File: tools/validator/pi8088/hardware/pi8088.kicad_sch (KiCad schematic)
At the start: 2 parts

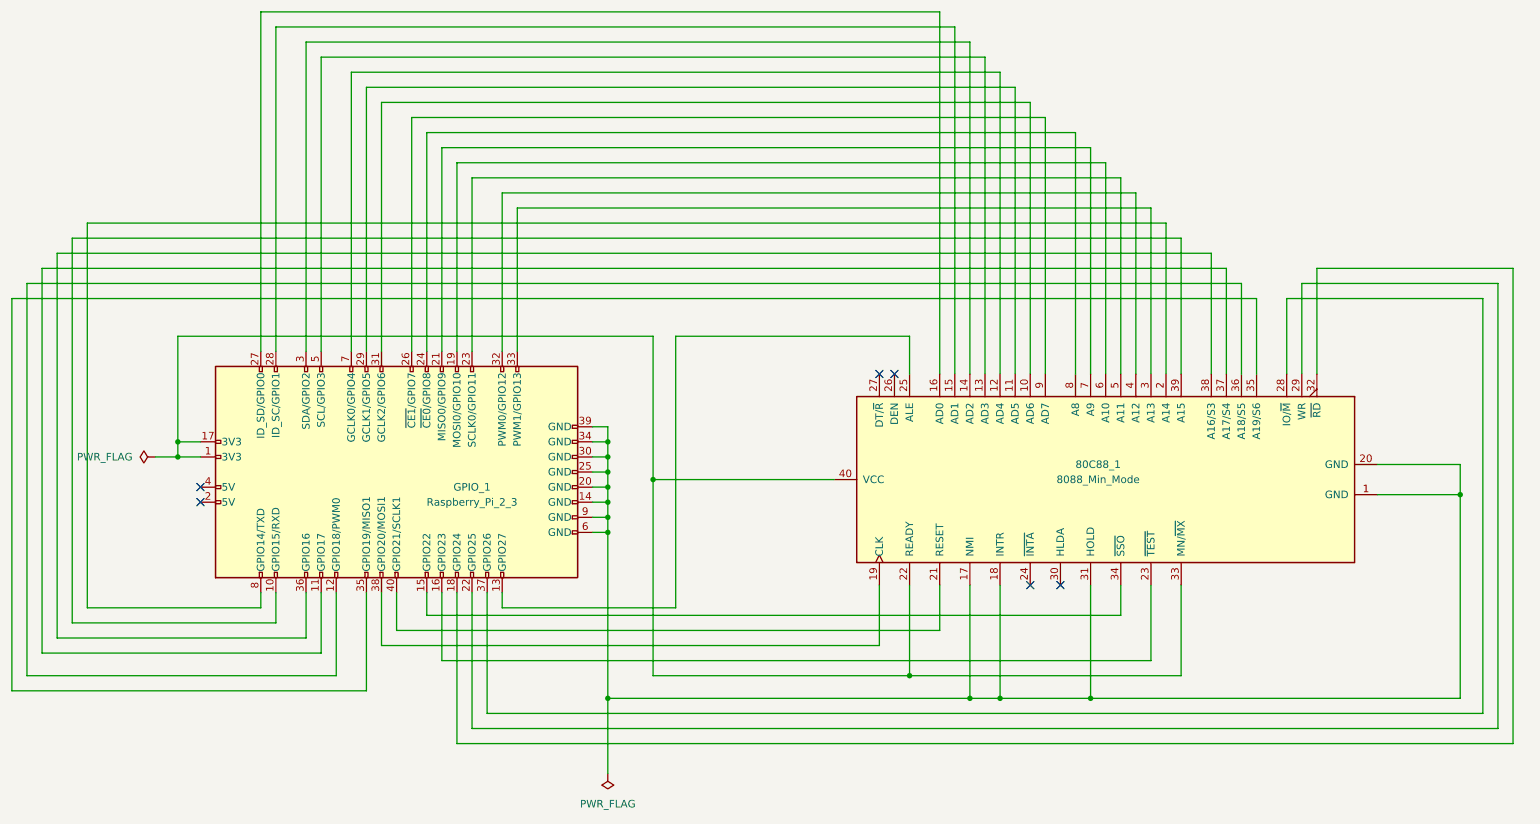
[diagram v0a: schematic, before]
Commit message: New pcb design
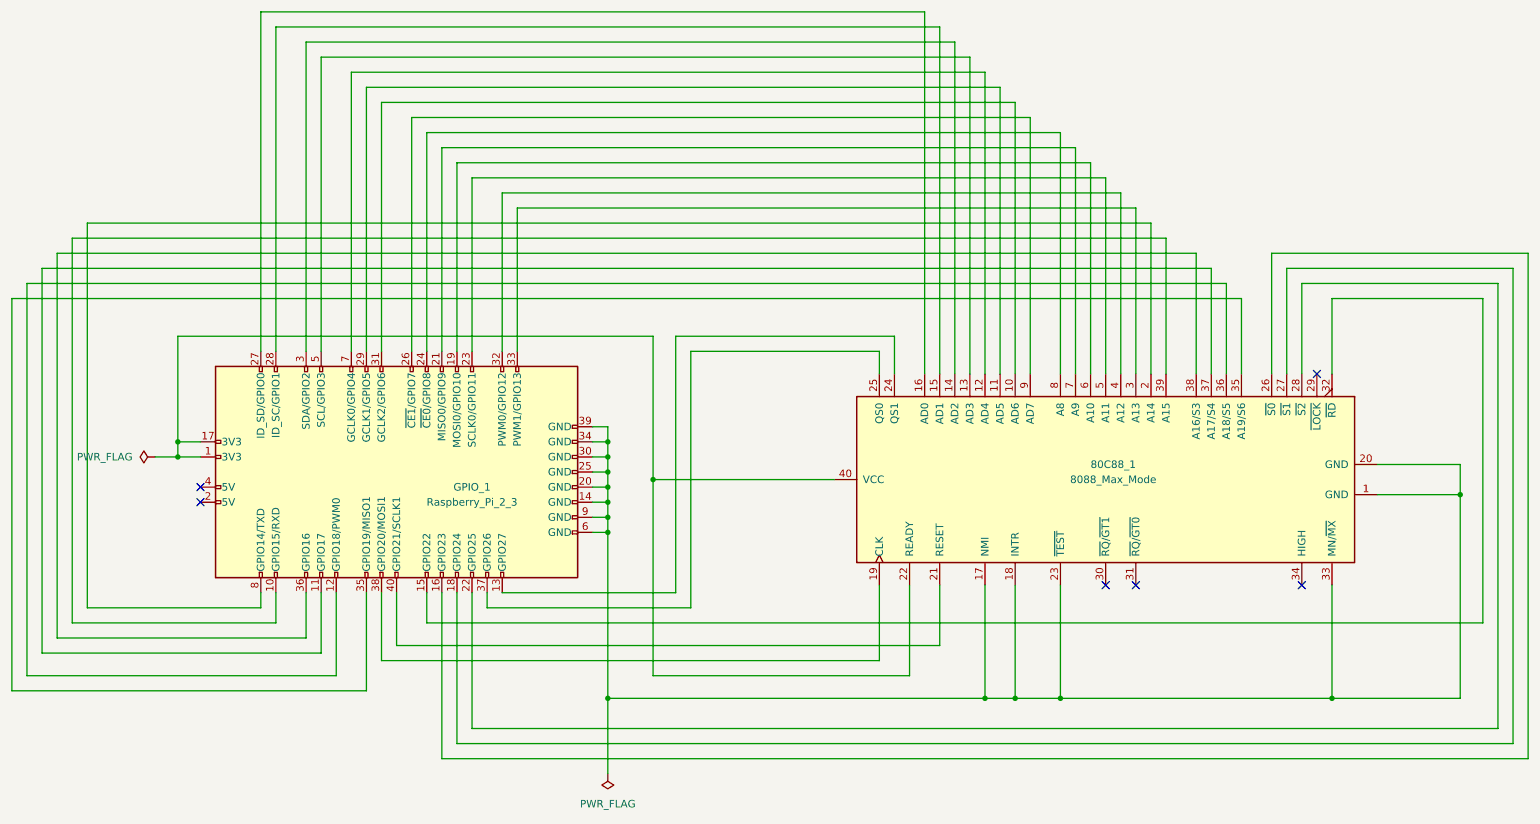
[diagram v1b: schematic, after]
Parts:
- removed 80C88_1: 8088_Min_Mode, Package_DIP:DIP-40_W15.24mm_Socket, symbol MCU_Intel:8088_Min_Mode
- added 80C88_1: 8088_Max_Mode, Package_DIP:DIP-40_W15.24mm, symbol MCU_Intel:8088_Max_Mode
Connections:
- net at GPIO_1.1 (3V3), GPIO_1.17 (3V3): now also 80C88_1.22 (READY), 80C88_1.40 (VCC)
- net at GPIO_1.10 (GPIO15/RXD): now also 80C88_1.39 (A15)
- net at GPIO_1.11 (GPIO17): now also 80C88_1.37 (A17/S4)
- net at GPIO_1.12 (GPIO18/PWM0): now also 80C88_1.36 (A18/S5)
- net at GPIO_1.13 (GPIO27): now also 80C88_1.24 (QS1)
- net at GPIO_1.14 (GND), GPIO_1.20 (GND), GPIO_1.25 (GND)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: now also 80C88_1.1 (GND), 80C88_1.17 (NMI), 80C88_1.18 (INTR), 80C88_1.20 (GND), 80C88_1.23 (~{TEST}), 80C88_1.33 (MN/~{MX})
- net at GPIO_1.15 (GPIO22): now also 80C88_1.32 (~{RD})
- net at GPIO_1.16 (GPIO23): now also 80C88_1.26 (~{S0})
- net at GPIO_1.18 (GPIO24): now also 80C88_1.27 (~{S1})
- net at GPIO_1.19 (MOSI0/GPIO10): now also 80C88_1.6 (A10)
- net at GPIO_1.21 (MISO0/GPIO9): now also 80C88_1.7 (A9)
- net at GPIO_1.22 (GPIO25): now also 80C88_1.28 (~{S2})
- net at GPIO_1.23 (SCLK0/GPIO11): now also 80C88_1.5 (A11)
- net at GPIO_1.24 (~{CE0}/GPIO8): now also 80C88_1.8 (A8)
- net at GPIO_1.26 (~{CE1}/GPIO7): now also 80C88_1.9 (AD7)
- net at GPIO_1.27 (ID_SD/GPIO0): now also 80C88_1.16 (AD0)
- net at GPIO_1.28 (ID_SC/GPIO1): now also 80C88_1.15 (AD1)
- net at GPIO_1.29 (GCLK1/GPIO5): now also 80C88_1.11 (AD5)
- net at GPIO_1.3 (SDA/GPIO2): now also 80C88_1.14 (AD2)
- net at GPIO_1.31 (GCLK2/GPIO6): now also 80C88_1.10 (AD6)
- net at GPIO_1.32 (PWM0/GPIO12): now also 80C88_1.4 (A12)
- net at GPIO_1.33 (PWM1/GPIO13): now also 80C88_1.3 (A13)
- net at GPIO_1.35 (GPIO19/MISO1): now also 80C88_1.35 (A19/S6)
- net at GPIO_1.36 (GPIO16): now also 80C88_1.38 (A16/S3)
- net at GPIO_1.37 (GPIO26): now also 80C88_1.25 (QS0)
- net at GPIO_1.38 (GPIO20/MOSI1): now also 80C88_1.19 (CLK)
- net at GPIO_1.40 (GPIO21/SCLK1): now also 80C88_1.21 (RESET)
- net at GPIO_1.5 (SCL/GPIO3): now also 80C88_1.13 (AD3)
- net at GPIO_1.7 (GCLK0/GPIO4): now also 80C88_1.12 (AD4)
- net at GPIO_1.8 (GPIO14/TXD): now also 80C88_1.2 (A14)
